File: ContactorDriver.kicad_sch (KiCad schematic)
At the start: 22 parts, among them Con1 LED, Con2 LED, J6 ContactorConnector, J7 ContactorConnector, Q2 IRLML0030, Q3 IRLML0030, U2 EL3H7, U3 EL3H7

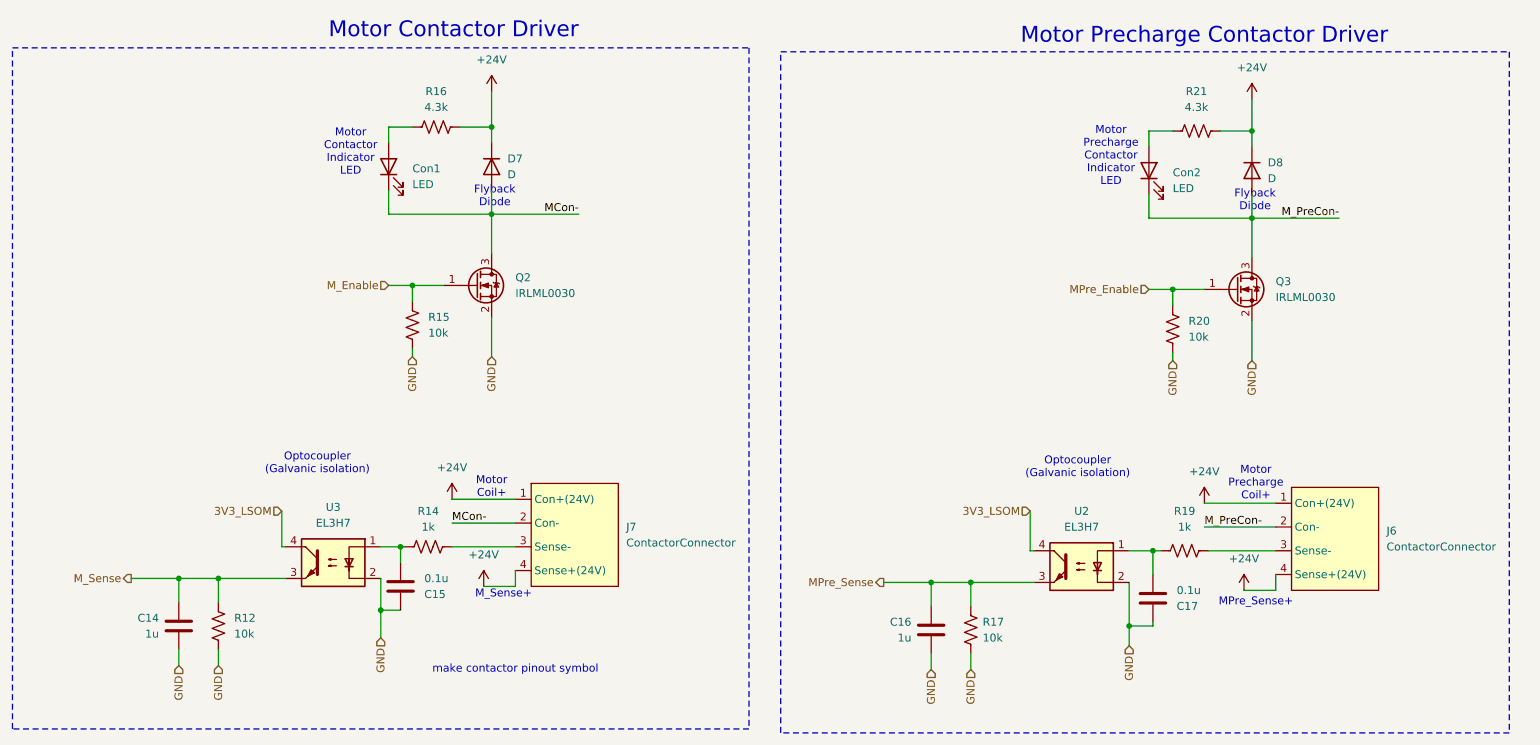
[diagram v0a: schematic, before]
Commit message: start of RevB. BOM for revA
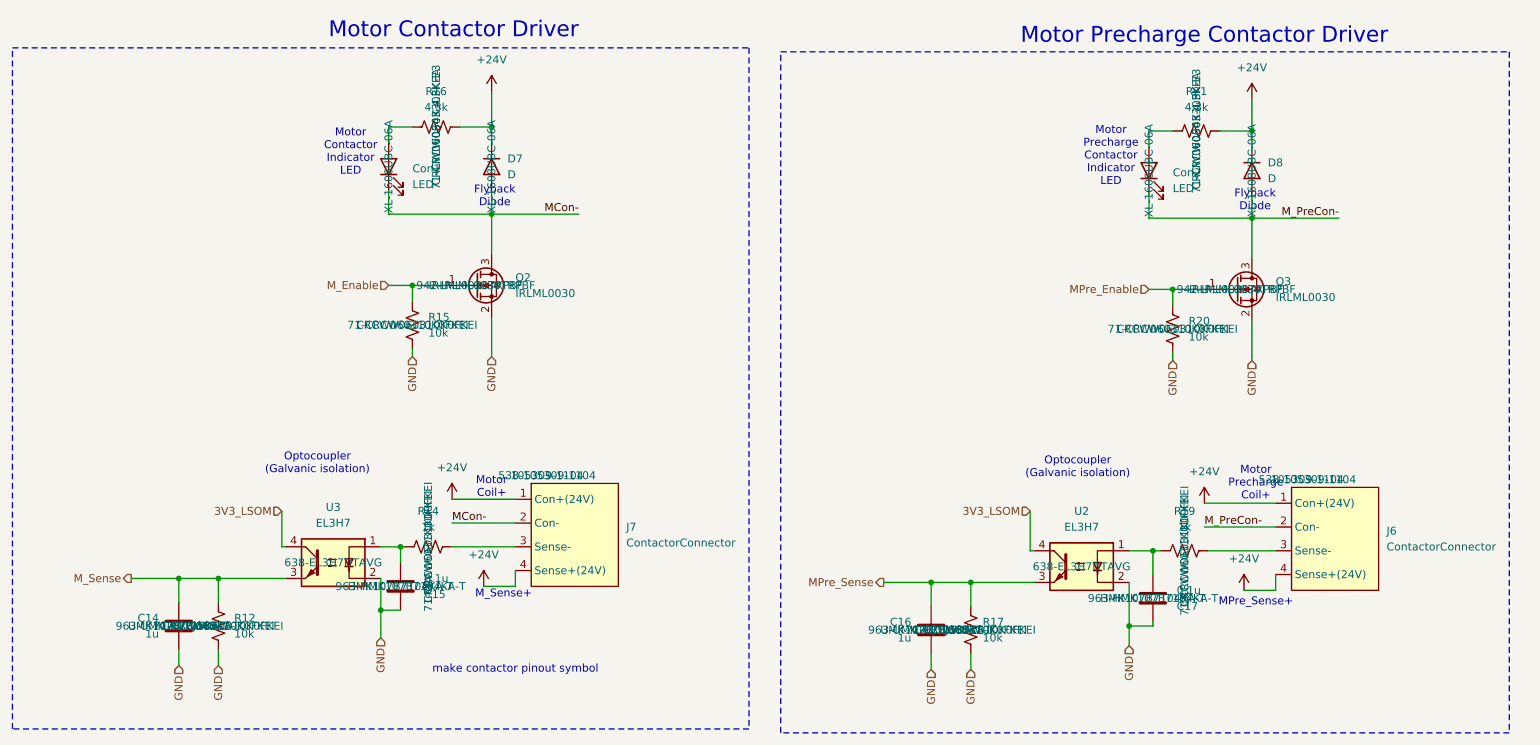
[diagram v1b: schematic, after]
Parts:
- C14, C16: Mouser Part Number (none) -> 963-UMK107BJ105KA-T; P/N (none) -> UMK107BJ105KA-T
- C15, C17: Mouser Part Number (none) -> 963-HMK107B7104KA-T; P/N (none) -> HMK107B7104KA-T
- Con1, Con2, D7, D8: P/N (none) -> XL-1608UBC-06A
- J6, J7: Mouser Part Number (none) -> 538-105309-1104; P/N (none) -> 105309-1104
- Q2, Q3: Mouser Part Number (none) -> 942-IRLML0030TRPBF; P/N (none) -> IRLML0030TRPBF
- R12, R15, R17, R20: Mouser Part Number (none) -> 71-CRCW060310K0FKEI; P/N (none) -> CRCW060310K0FKEI
- R14, R19: Mouser Part Number (none) -> 71-CRCW06031K00FKEI; P/N (none) -> CRCW06031K00FKEI
- R16, R21: Mouser Part Number (none) -> 71-CRCW0603-4.3K-E3; P/N (none) -> CRCW06034K30FKEA
- U2, U3: Mouser Part Number (none) -> 638-EL3H7DTAVG
